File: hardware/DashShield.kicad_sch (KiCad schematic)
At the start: 60 parts, among them J1 GPIO, J2 Steering Wheel, J3 Dash LEDs, J4 CAN 0, J5 PWR, J6 CAN 1, Q1 2N7002, Q2 2N7002, Q3 2N7002, Q4 2N7002, Q5 2N7002, Q6 2N7002, U1 CAT24C256, U2 MCP2562-E-SN, U3 MCP2515-xST, U4 MCP2515-xST, U5 MCP2562-E-SN, Y1 8MHz, Y2 8MHz

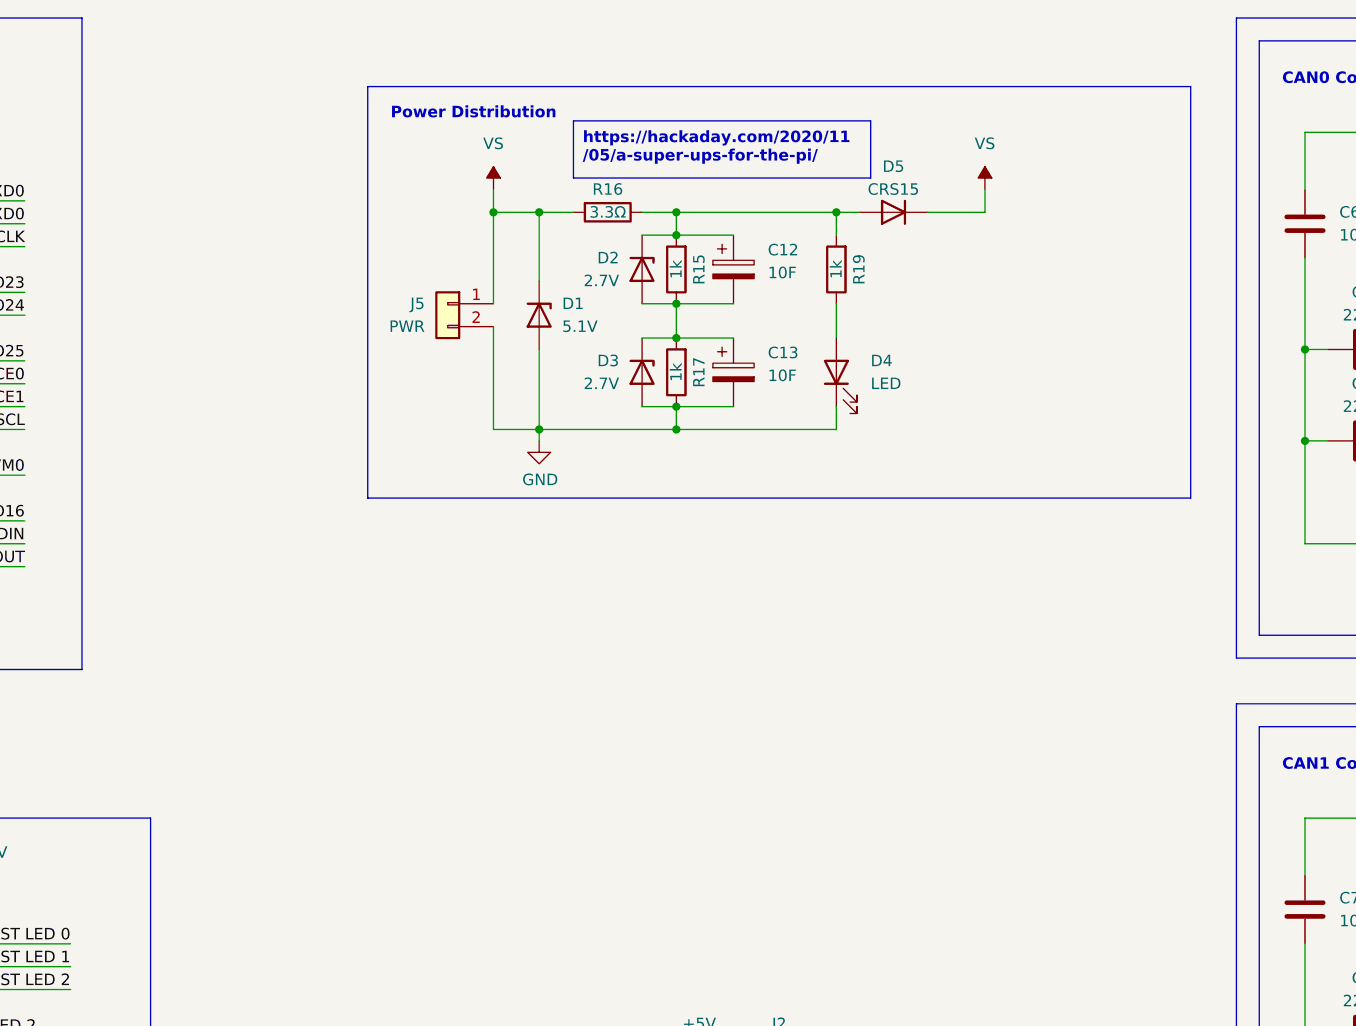
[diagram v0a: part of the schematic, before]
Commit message: feat: finish power supply
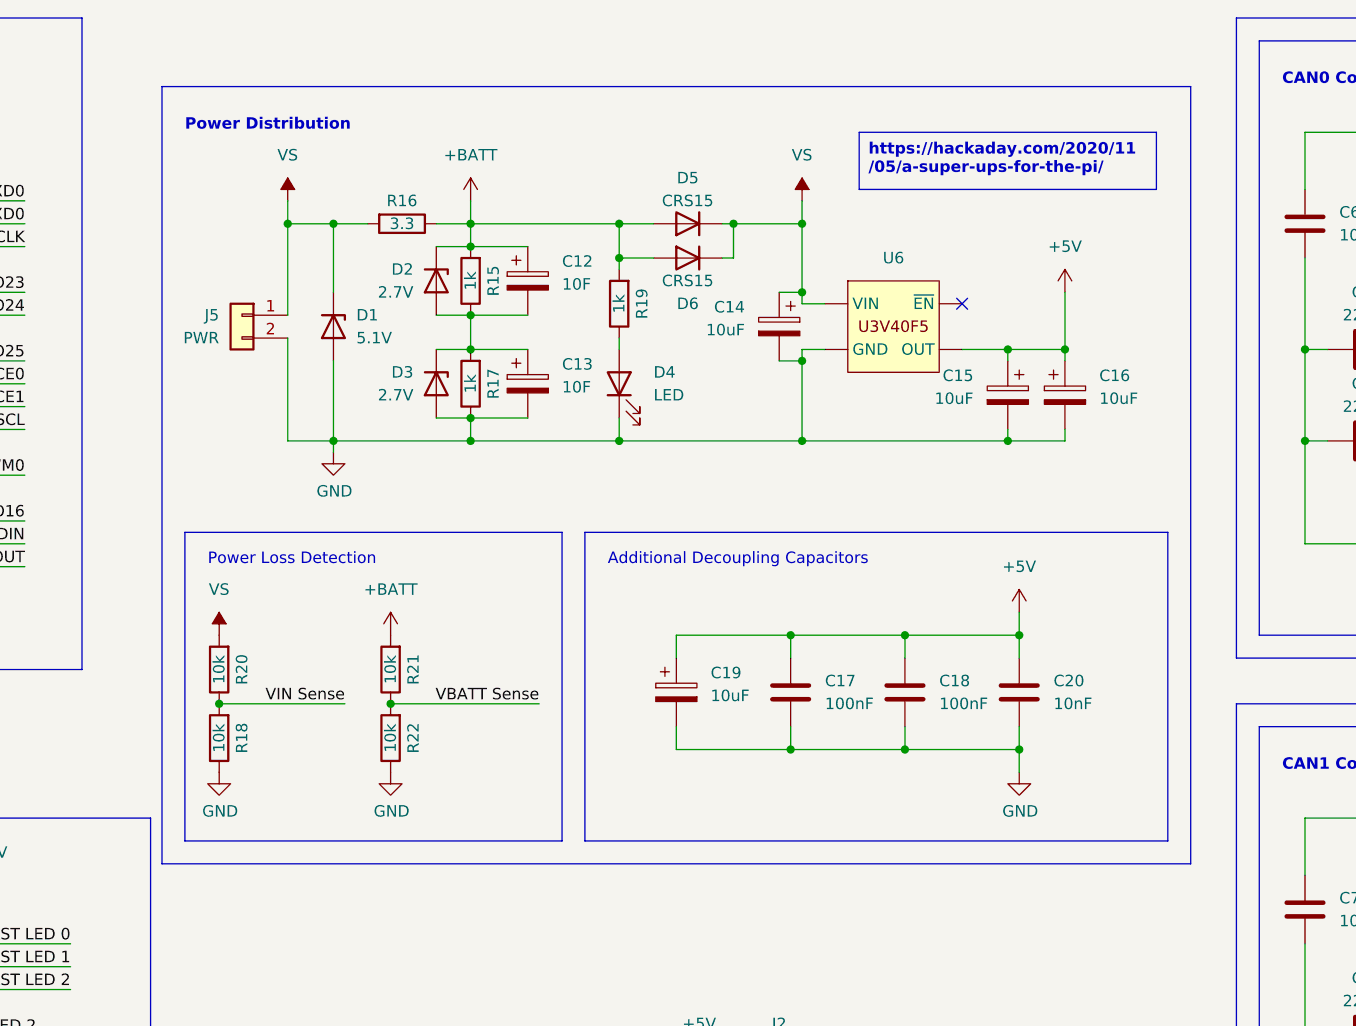
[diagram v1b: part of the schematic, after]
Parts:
- added C14, C15, C16, C19: 10uF, symbol Device:C_Polarized
- added C17, C18: 100nF, symbol Device:C
- added C20: 10nF, symbol Device:C
- added D6: CRS15, Diode_SMD:D_SOD-123F, symbol Device:D
- added R18, R20, R21, R22: 10k, symbol Device:R
- added U6: ~, U3V40x:U3V40x, symbol U3V40x:U3V40F5
- R16: value 3.3Ω -> 3.3
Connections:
- net +5V: now also C15.1, C16.1, C17.1, C18.1, C19.1, C20.1, U6. (~{EN})
- net GND: now also C14.2, C15.2, C16.2, C17.2, C18.2, C19.2, C20.2, R18.1, R22.1, U6. (~{EN})
- net VS: now also C14.1, D6.1 (K), R20.2, U6. (~{EN})
- net +BATT: now reaches C12.1, D2.1 (K), D5.2 (A), R15.2, R16.1, R19.2
- net +BATT: now also D6.2 (A), R21.2
- new net VBATT Sense: R21.1, R22.2
- new net VIN Sense: R18.2, R20.1
- no-connect marks 15 -> 16
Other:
- note added: "Additional Decoupling Capacitors"
- note added: "Power Loss Detection"
- moved on the sheet: C12, C13, D1, D2, D3, D4, D5, J5, R15, R16, R17, R19
